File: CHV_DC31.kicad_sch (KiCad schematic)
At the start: 92 parts, among them IC1 W25Q16JVUXIQ_TR, J1 USB_C_Receptacle_USB2.0, J2 Conn_01x02, J3 Conn_02x03_Odd_Even, J4 Conn_02x03_Odd_Even, J5 Conn_02x03_Odd_Even, J6 Conn_01x03, U1 MCP2558FD-xMNY, U2 XC6220B331MR, U3 RP2040, U4 MCP2558FD-xMNY, U5 MCP2558FD-xMNY, U6 MCP2558FD-xMNY, Y1 XYDBPCNANF-12MHz

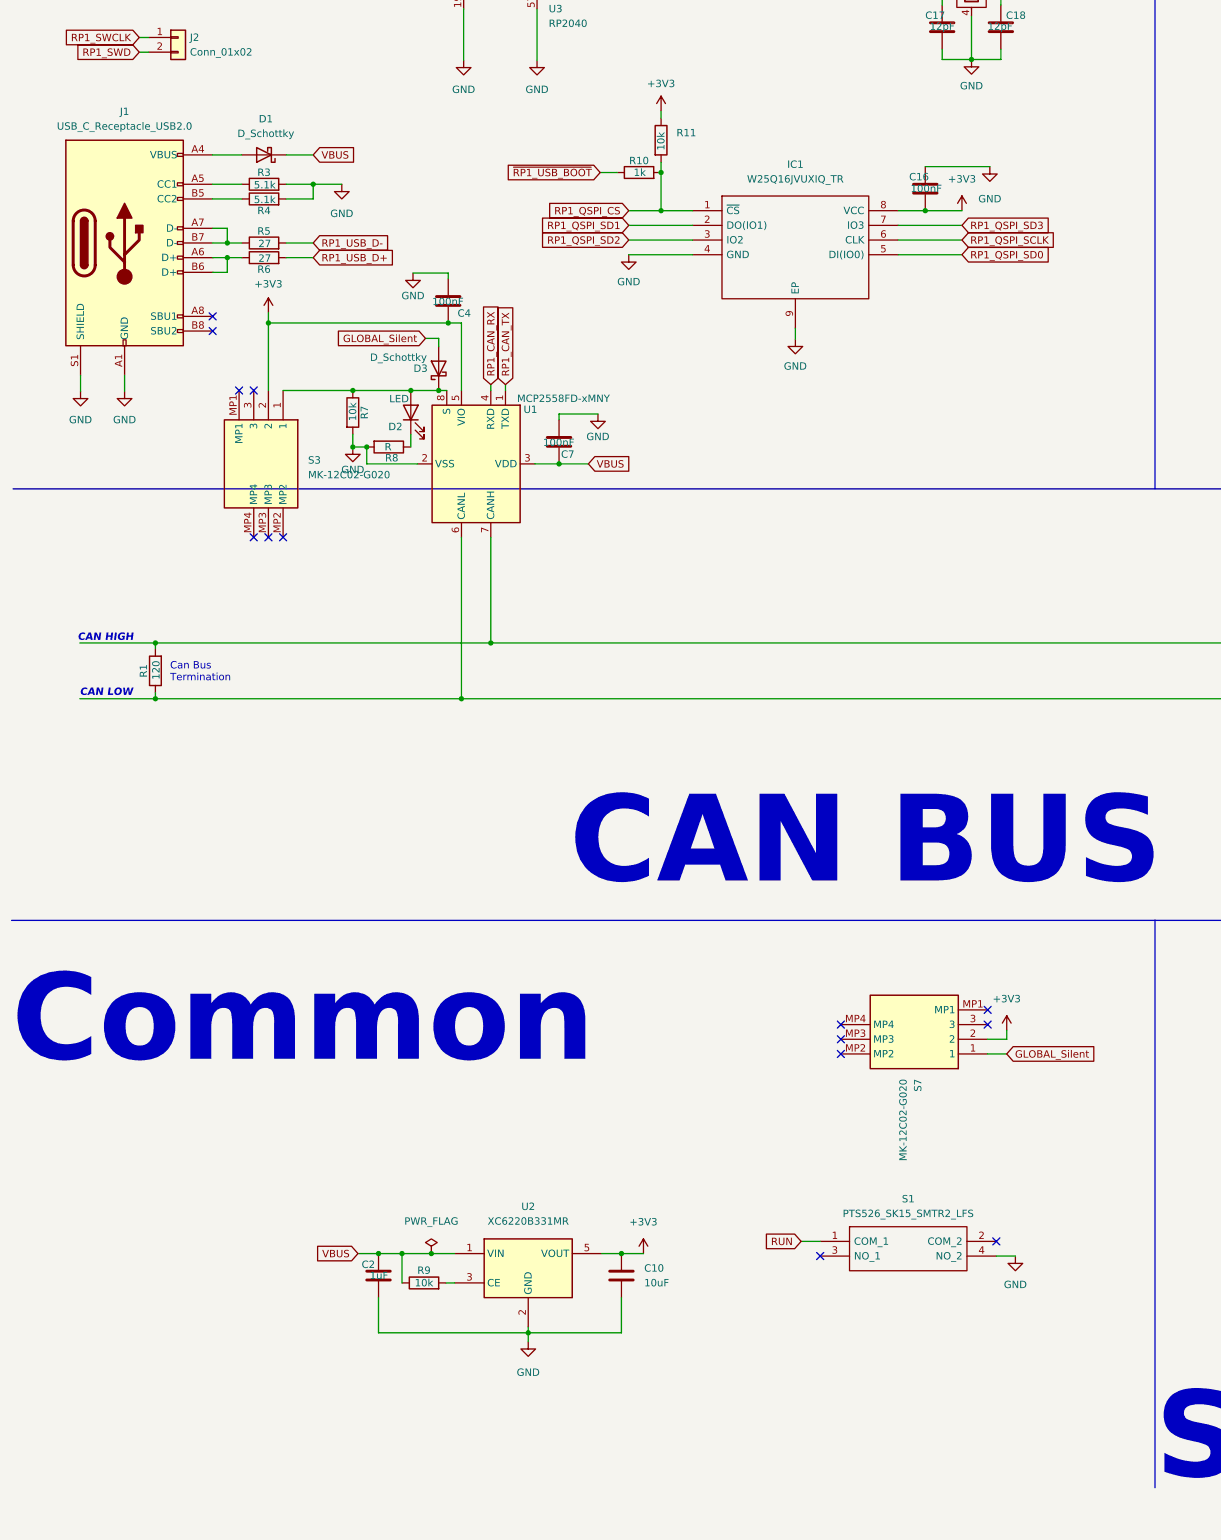
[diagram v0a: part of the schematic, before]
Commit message: getting closer
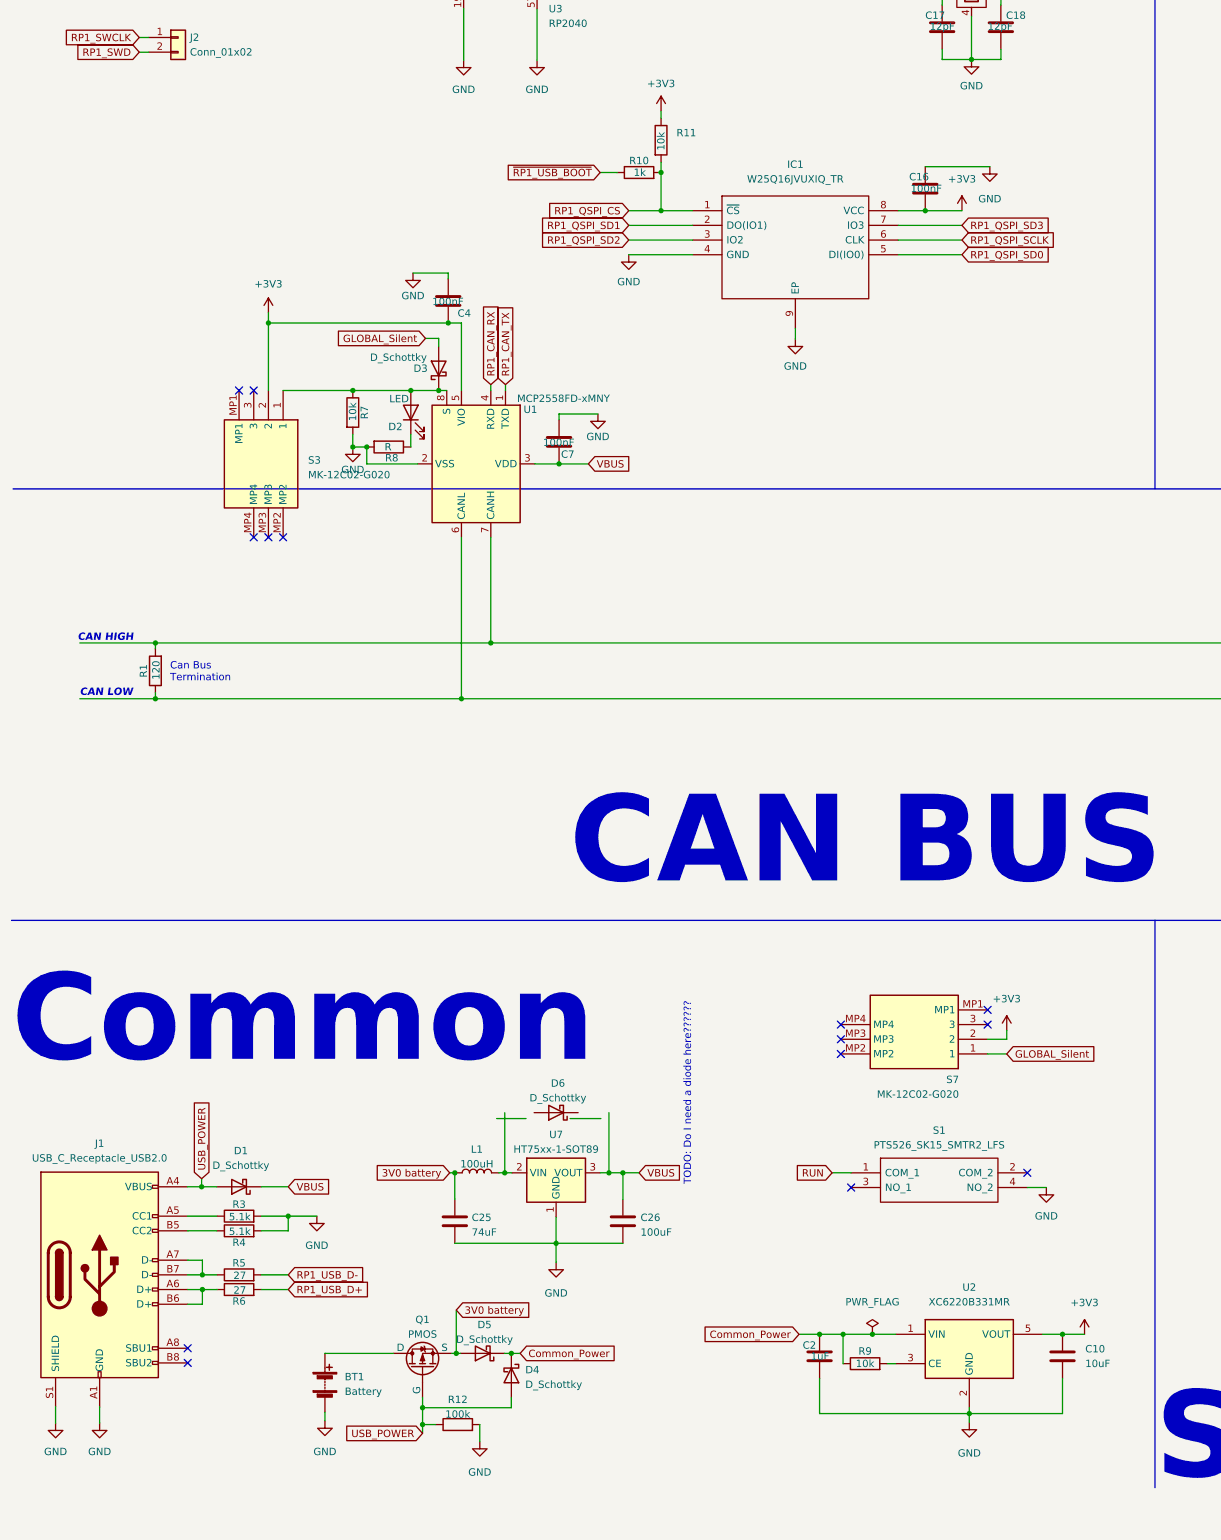
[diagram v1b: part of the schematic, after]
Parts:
- added BT1: Battery, symbol Device:Battery
- added C25: 74uF, symbol Device:C
- added C26: 100uF, symbol Device:C
- added D4, D5: D_Schottky, Diode_SMD:D_SOD-123, symbol Device:D_Schottky
- added D6: D_Schottky, symbol Device:D_Schottky
- added L1: 100uH, symbol Device:L
- added Q1: PMOS, symbol Simulation_SPICE:PMOS
- added R12: 100k, symbol Device:R
- added U7: HT75xx-1-SOT89, Package_TO_SOT_SMD:SOT-89-3, symbol Regulator_Linear:HT75xx-1-SOT89
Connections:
- net GND: now also BT1.2 (-), C25.2, C26.2, R12.2, U7.1 (GND)
- net VBUS: now also C26.1, U7.3 (VOUT); no longer C2.1, R9.1, U2.1 (VIN)
- net USB_POWER: now reaches D1.2 (A), J1.A4 (VBUS), J1.A9 (VBUS), J1.B4 (VBUS), J1.B9 (VBUS)
- net USB_POWER: now also D4.2 (A), Q1.2 (G), R12.1
- new net: L1.2, U7.2 (VIN)
- new net: BT1.1 (+), Q1.1 (D)
- new net 3V0 battery: C25.1, D5.2 (A), L1.1, Q1.3 (S)
- new net Common_Power: C2.1, D4.1 (K), D5.1 (K), R9.1, U2.1 (VIN)
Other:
- note added: "TODO: Do I need a diode here??????"
- moved on the sheet: C10, C2, D1, J1, R3, R4, R5, R6, R9, S1, U2
